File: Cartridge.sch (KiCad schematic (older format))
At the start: 3 parts, among them J24 Cartridge, J4 Expansion

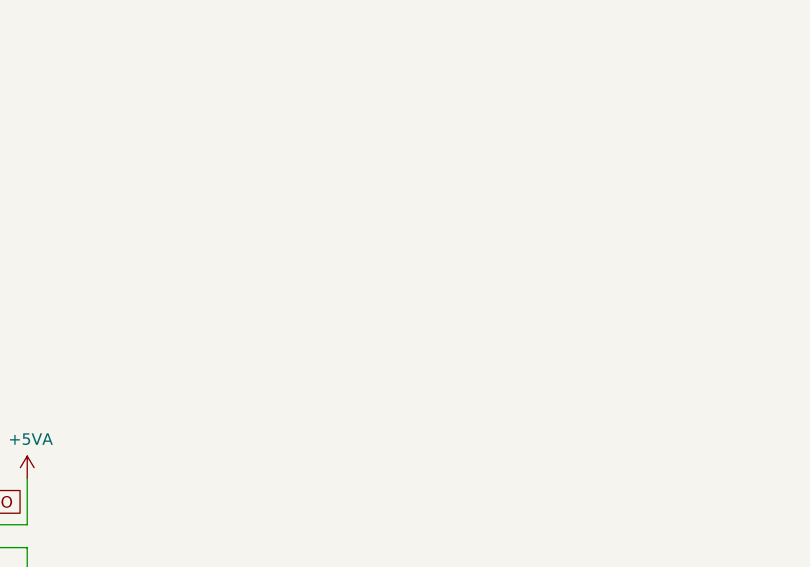
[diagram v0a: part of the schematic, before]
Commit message: Diagnostic
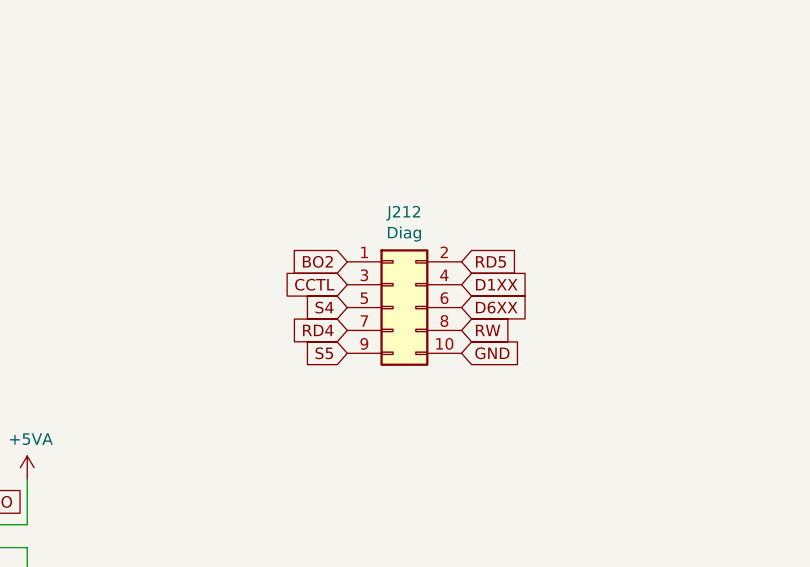
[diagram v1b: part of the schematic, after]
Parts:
- added J212: Diag, Connector_PinHeader_2.54mm:PinHeader_2x05_P2.54mm_Vertical, symbol Connector_Generic:Conn_02x05_Odd_Even
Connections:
- net BO2: now also J212.1 (Pin_1)
- net CCTL: now also J212.3 (Pin_3)
- net D1XX: now also J212.4 (Pin_4)
- net GND: now also J212.10 (Pin_10)
- net RD4: now also J212.7 (Pin_7)
- net RD5: now also J212.2 (Pin_2)
- net RW: now also J212.8 (Pin_8)
- net S4: now also J212.5 (Pin_5)
- net S5: now also J212.9 (Pin_9)
- new net D6XX: J212.6 (Pin_6)
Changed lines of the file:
@@
+	1    0    0    -1
+$EndComp
+Text GLabel 5025 2900 2    50   Input ~ 0
+D1XX
+Text GLabel 4525 2800 0    50   Input ~ 0
+BO2
+Text GLabel 4525 2900 0    50   Input ~ 0
+CCTL
+Text GLabel 4525 3000 0    50   Input ~ 0
+S4
+Text GLabel 4525 3100 0    50   Input ~ 0
+RD4
+Text GLabel 4525 3200 0    50   Input ~ 0
+S5
+Text GLabel 5025 2800 2    50   Input ~ 0
+RD5
+Text GLabel 5025 3000 2    50   Input ~ 0
+D6XX
+Text GLabel 5025 3200 2    50   Input ~ 0
+GND
+Text GLabel 5025 3100 2    50   Input ~ 0
+RW
+$Comp
+L Connector_Generic:Conn_02x05_Odd_Even J212
+U 1 1 604245DE
+P 4725 3000
+F 0 "J212" H 4775 3417 50  0000 C CNN
+F 1 "Diag" H 4775 3326 50  0000 C CNN
+F 2 "Connector_PinHeader_2.54mm:PinHeader_2x05_P2.54mm_Vertical" H 4725 3000 50  0001 C CNN
+F 3 "~" H 4725 3000 50  0001 C CNN
+	1    4725 3000
 	1    0    0    -1
 $EndComp
